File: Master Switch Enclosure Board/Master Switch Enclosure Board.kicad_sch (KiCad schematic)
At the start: 14 parts, among them J1 Harness In A, J2 Harness In B, J3 Harness Out, J4 Screw_Terminal_01x04, J5 Screw_Terminal_01x04, J6 20-pin MicroFit, J7 4-pin MicroFit

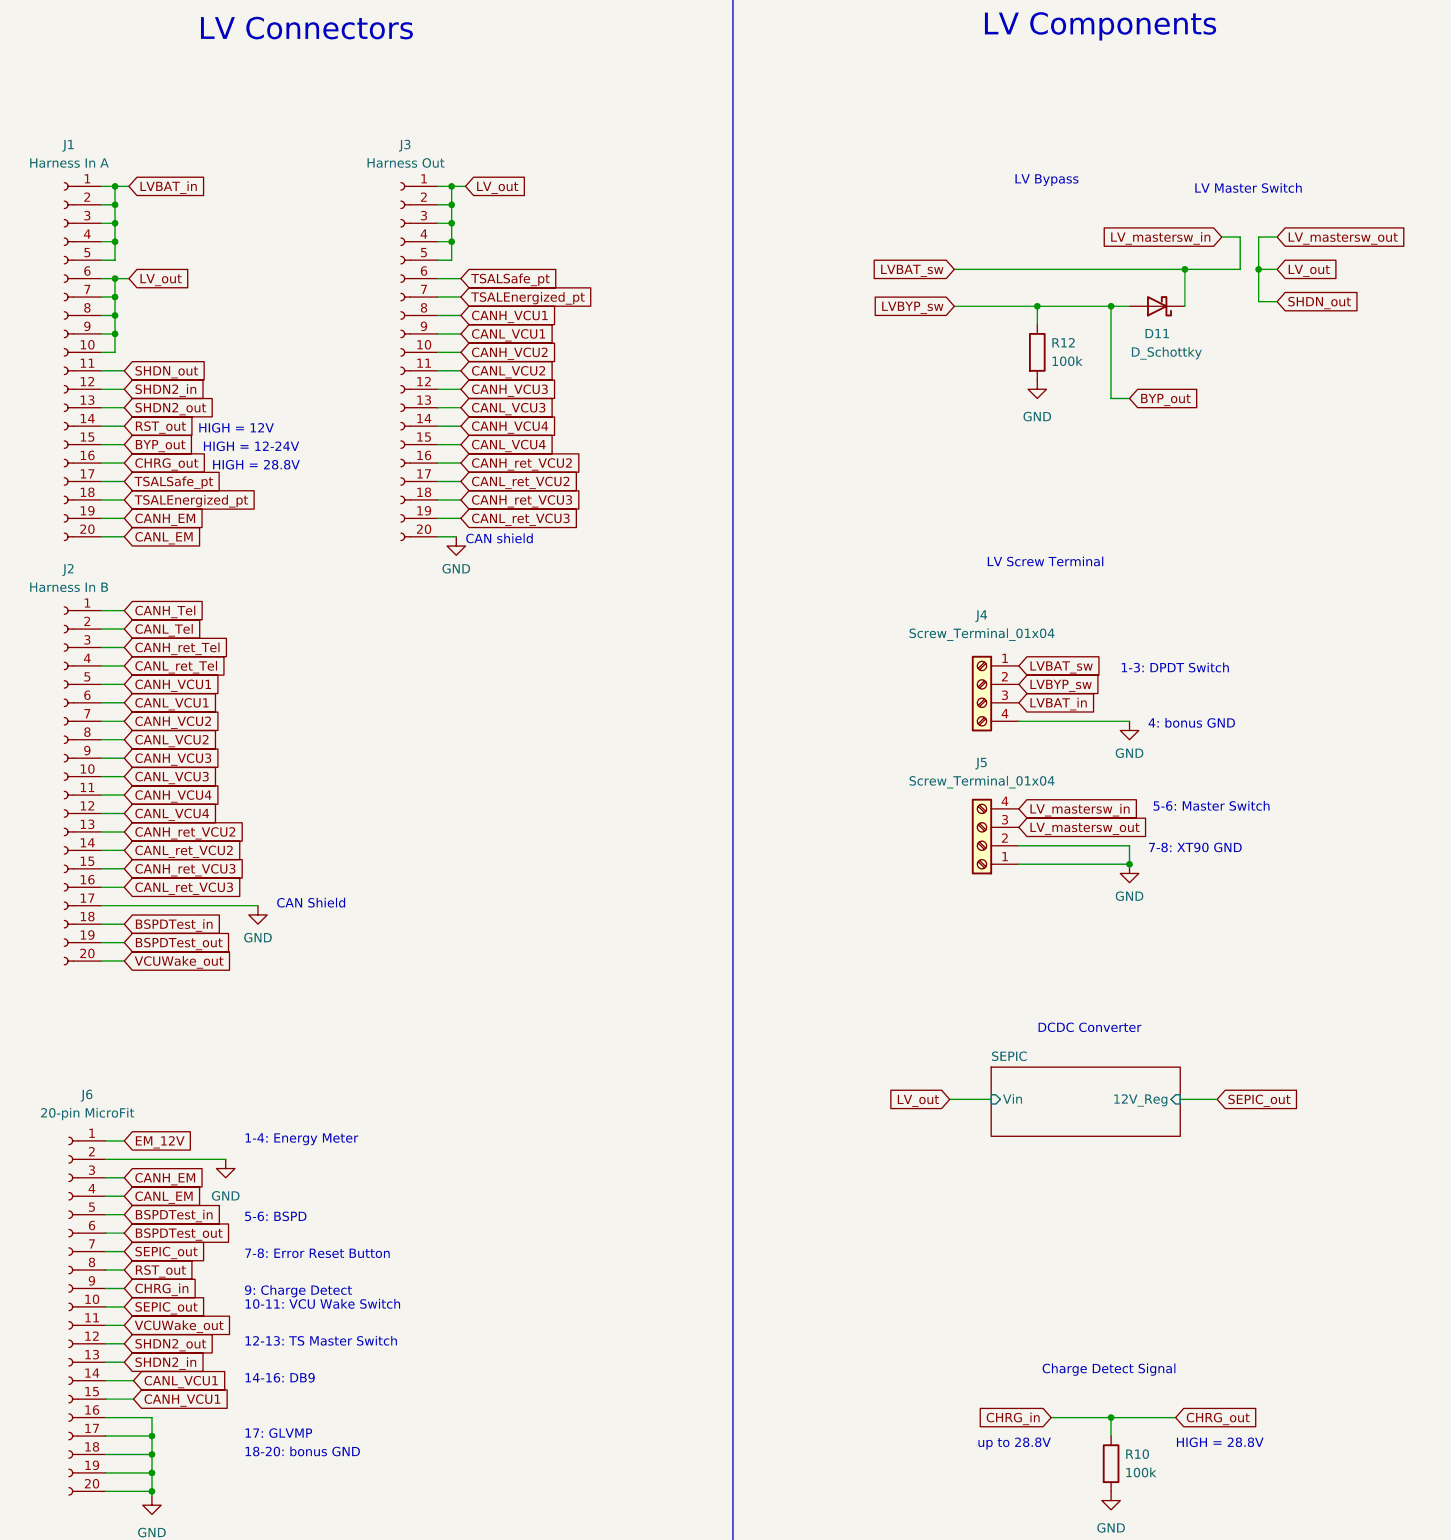
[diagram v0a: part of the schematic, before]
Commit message: finished routing
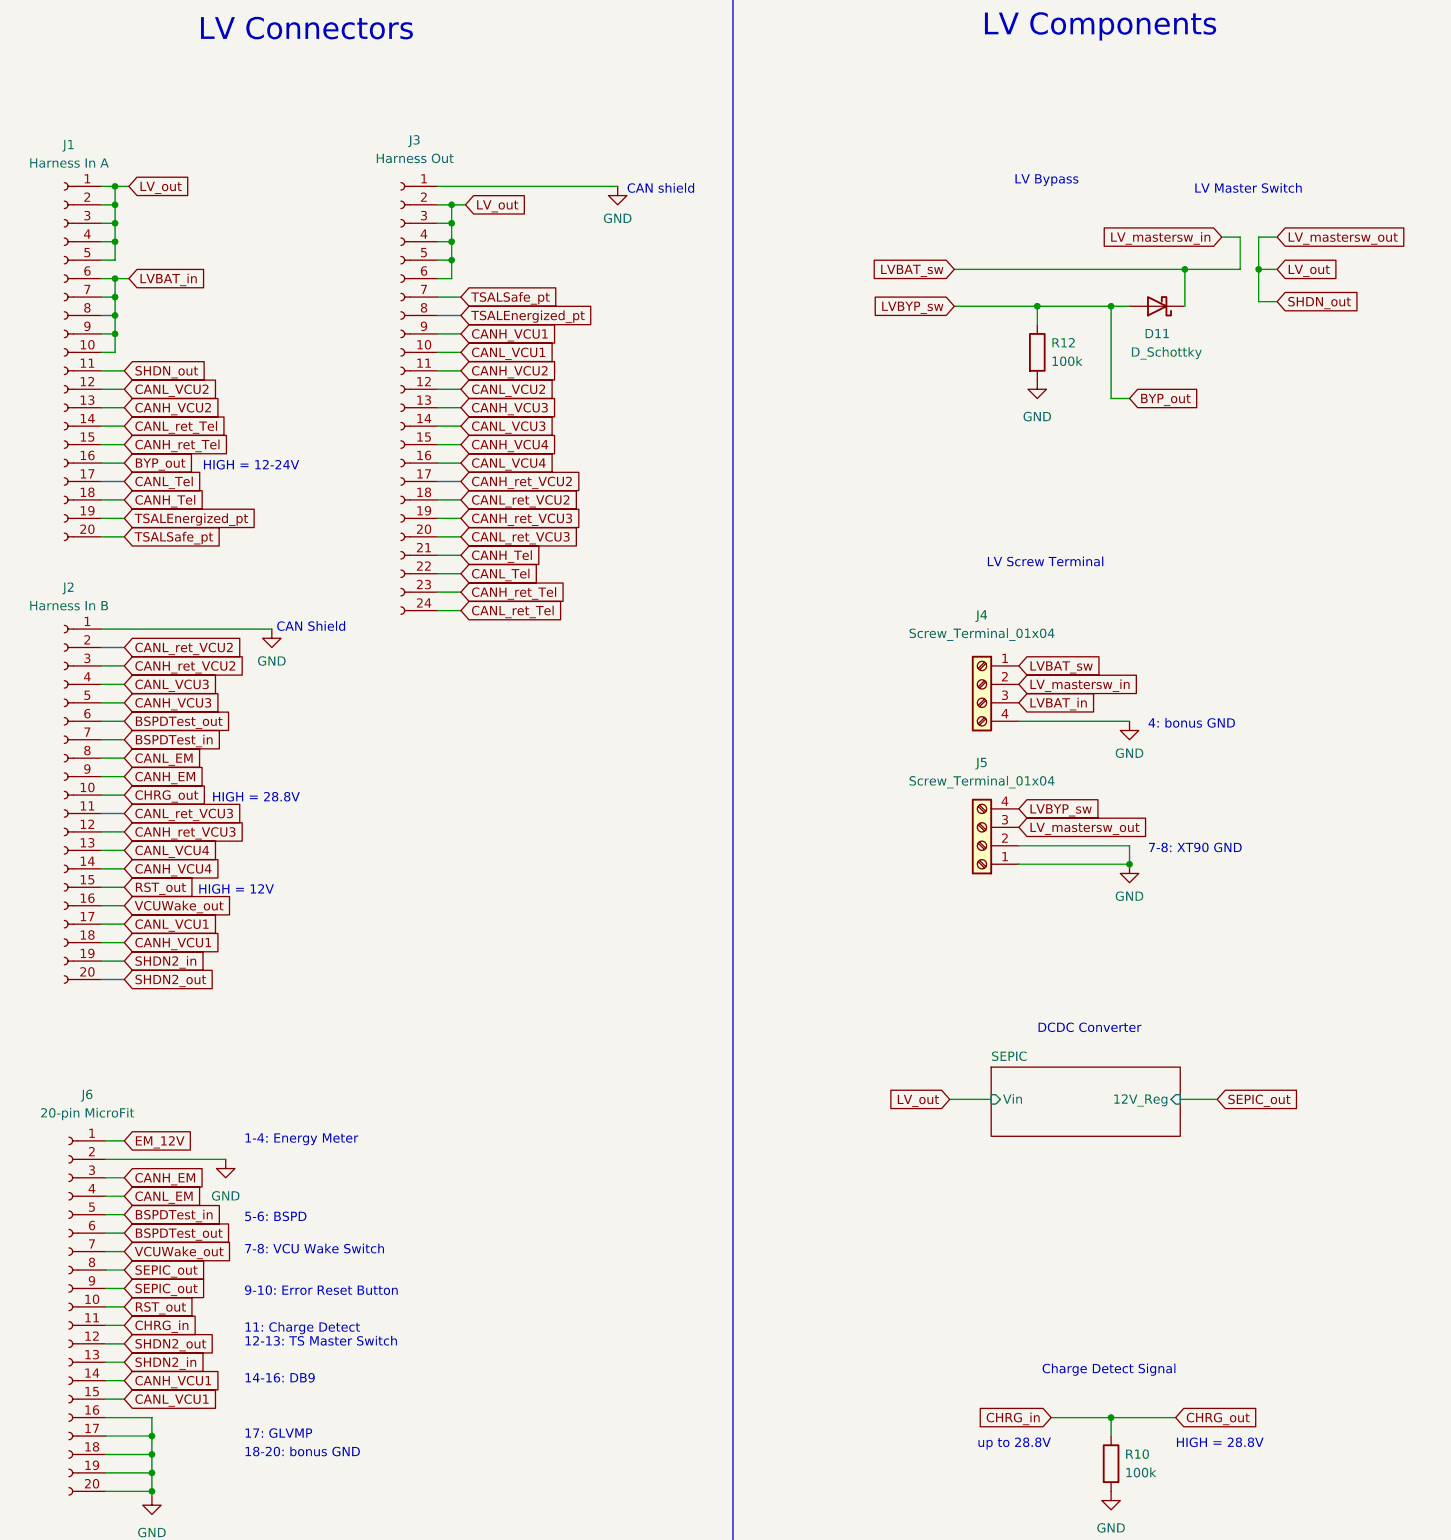
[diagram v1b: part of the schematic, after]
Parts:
- removed J3: Harness Out, Connector_Molex:Molex_Micro-Fit_3.0_43045-2012_2x10_P3.00mm_Vertical, symbol Connector:Conn_01x20_Female
- added J3: Harness Out, Connector_Molex:Molex_Micro-Fit_3.0_43045-2412_2x12_P3.00mm_Vertical, symbol Connector:Conn_01x24_Female
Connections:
- net BSPDTest_in: now also J2.7 (Pin_7); no longer J2.18 (Pin_18)
- net BSPDTest_out: now also J2.6 (Pin_6); no longer J2.19 (Pin_19)
- net BYP_out: now also J1.16 (Pin_16), J5.4 (Pin_4); no longer J1.15 (Pin_15), J4.2 (Pin_2)
- net CANH_EM: now also J2.9 (Pin_9); no longer J1.19 (Pin_19)
- net CANH_Tel: now also J1.18 (Pin_18), J3.21 (Pin_21); no longer J2.1 (Pin_1)
- net CANH_VCU1: now also J2.18 (Pin_18), J6.14 (Pin_14), J3.9 (Pin_9); no longer J2.5 (Pin_5), J6.15 (Pin_15)
- net CANH_VCU2: now also J1.13 (Pin_13), J3.11 (Pin_11); no longer J2.7 (Pin_7)
- net CANH_VCU3: now also J2.5 (Pin_5), J3.13 (Pin_13); no longer J2.9 (Pin_9)
- net CANH_VCU4: now also J2.14 (Pin_14), J3.15 (Pin_15); no longer J2.11 (Pin_11)
- net CANH_ret_Tel: now also J1.15 (Pin_15), J3.23 (Pin_23); no longer J2.3 (Pin_3)
- net CANH_ret_VCU2: now also J2.3 (Pin_3), J3.17 (Pin_17); no longer J2.13 (Pin_13)
- net CANH_ret_VCU3: now also J2.12 (Pin_12), J3.19 (Pin_19); no longer J2.15 (Pin_15)
- net CANL_EM: now also J2.8 (Pin_8); no longer J1.20 (Pin_20)
- net CANL_Tel: now also J1.17 (Pin_17), J3.22 (Pin_22); no longer J2.2 (Pin_2)
- net CANL_VCU1: now also J2.17 (Pin_17), J6.15 (Pin_15), J3.10 (Pin_10); no longer J2.6 (Pin_6), J6.14 (Pin_14)
- net CANL_VCU2: now also J1.12 (Pin_12), J3.12 (Pin_12); no longer J2.8 (Pin_8)
- net CANL_VCU3: now also J2.4 (Pin_4), J3.14 (Pin_14); no longer J2.10 (Pin_10)
- net CANL_VCU4: now also J2.13 (Pin_13), J3.16 (Pin_16); no longer J2.12 (Pin_12)
- net CANL_ret_Tel: now also J1.14 (Pin_14), J3.24 (Pin_24); no longer J2.4 (Pin_4)
- net CANL_ret_VCU2: now also J2.2 (Pin_2), J3.18 (Pin_18); no longer J2.14 (Pin_14)
- net CANL_ret_VCU3: now also J2.11 (Pin_11), J3.20 (Pin_20); no longer J2.16 (Pin_16)
- net CHRG_in: now also J2.10 (Pin_10), J6.11 (Pin_11); no longer J1.16 (Pin_16), J6.9 (Pin_9)
- net GND: now also J2.1 (Pin_1), J3.1 (Pin_1); no longer J2.17 (Pin_17)
- net LVBAT_in: now also J1.10 (Pin_10), J1.6 (Pin_6), J1.7 (Pin_7), J1.8 (Pin_8), J1.9 (Pin_9); no longer J1.1 (Pin_1), J1.2 (Pin_2), J1.3 (Pin_3), J1.4 (Pin_4), J1.5 (Pin_5)
- net LVBAT_sw: now also J4.2 (Pin_2); no longer J5.4 (Pin_4)
- net LV_mastersw_out: now also J1.1 (Pin_1), J1.2 (Pin_2), J1.3 (Pin_3), J1.4 (Pin_4), J1.5 (Pin_5), J3.2 (Pin_2), J3.3 (Pin_3), J3.4 (Pin_4), J3.5 (Pin_5), J3.6 (Pin_6); no longer J1.10 (Pin_10), J1.6 (Pin_6), J1.7 (Pin_7), J1.8 (Pin_8), J1.9 (Pin_9)
- net RST_out: now also J2.15 (Pin_15), J6.10 (Pin_10); no longer J1.14 (Pin_14), J6.8 (Pin_8)
- net SEPIC_out: now also J6.8 (Pin_8), J6.9 (Pin_9); no longer J6.10 (Pin_10), J6.7 (Pin_7)
- net SHDN2_in: now also J2.19 (Pin_19); no longer J1.12 (Pin_12)
- net SHDN2_out: now also J2.20 (Pin_20); no longer J1.13 (Pin_13)
- net TSALEnergized_pt: now also J1.19 (Pin_19), J3.8 (Pin_8); no longer J1.18 (Pin_18)
- net TSALSafe_pt: now also J1.20 (Pin_20), J3.7 (Pin_7); no longer J1.17 (Pin_17)
- net VCUWake_out: now also J2.16 (Pin_16), J6.7 (Pin_7); no longer J2.20 (Pin_20), J6.11 (Pin_11)
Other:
- note added: "11: Charge Detect"
- note added: "7-8: VCU Wake Switch"
- note added: "9-10: Error Reset Button"
- note removed: "1-3: DPDT Switch"
- note removed: "10-11: VCU Wake Switch"
- note removed: "5-6: Master Switch"
- note removed: "7-8: Error Reset Button"
- note removed: "9: Charge Detect"
- moved on the sheet: J2
